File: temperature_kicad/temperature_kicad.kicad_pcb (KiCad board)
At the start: 2 copper layers, 35.6 x 30.5 mm, 13 parts, among them U1 nRF24L01, U2 DS18B20, U3 LD2980, U4 ATTINY13A-PU

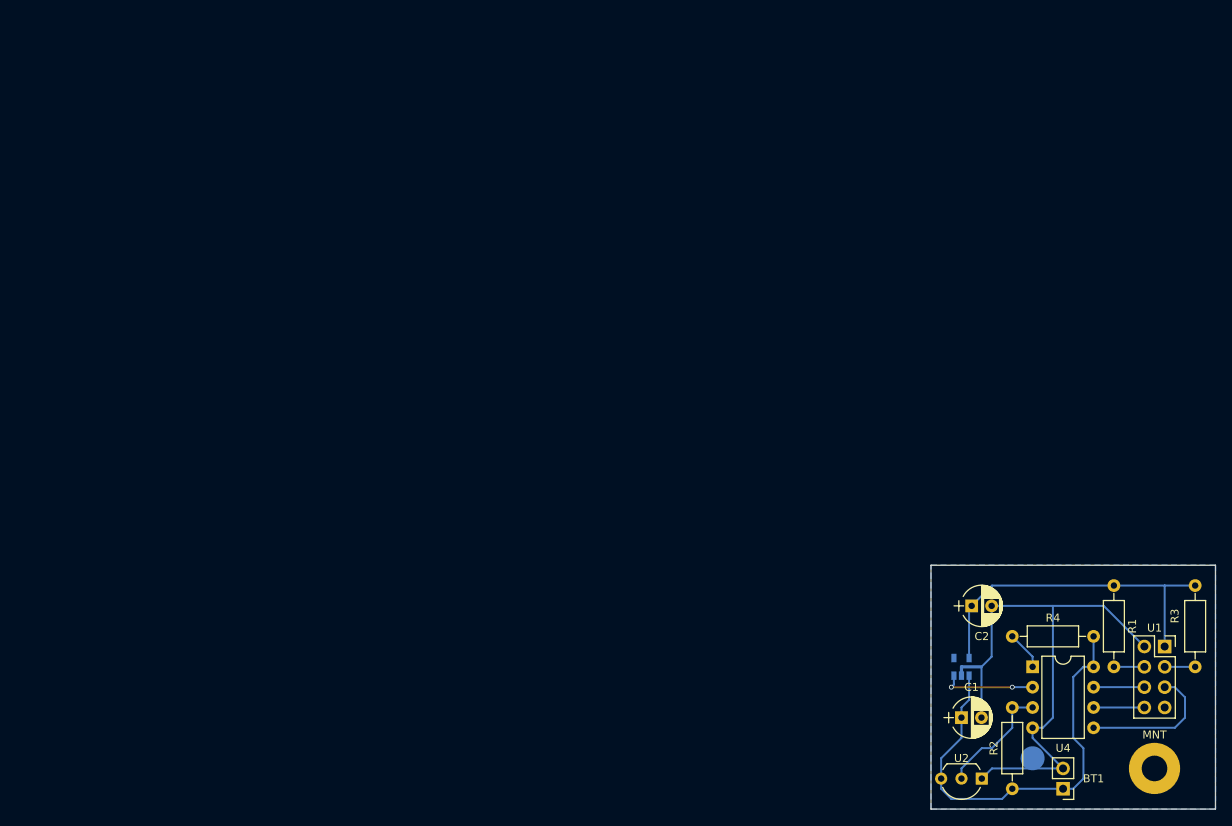
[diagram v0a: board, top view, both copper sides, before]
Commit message: Redone routing
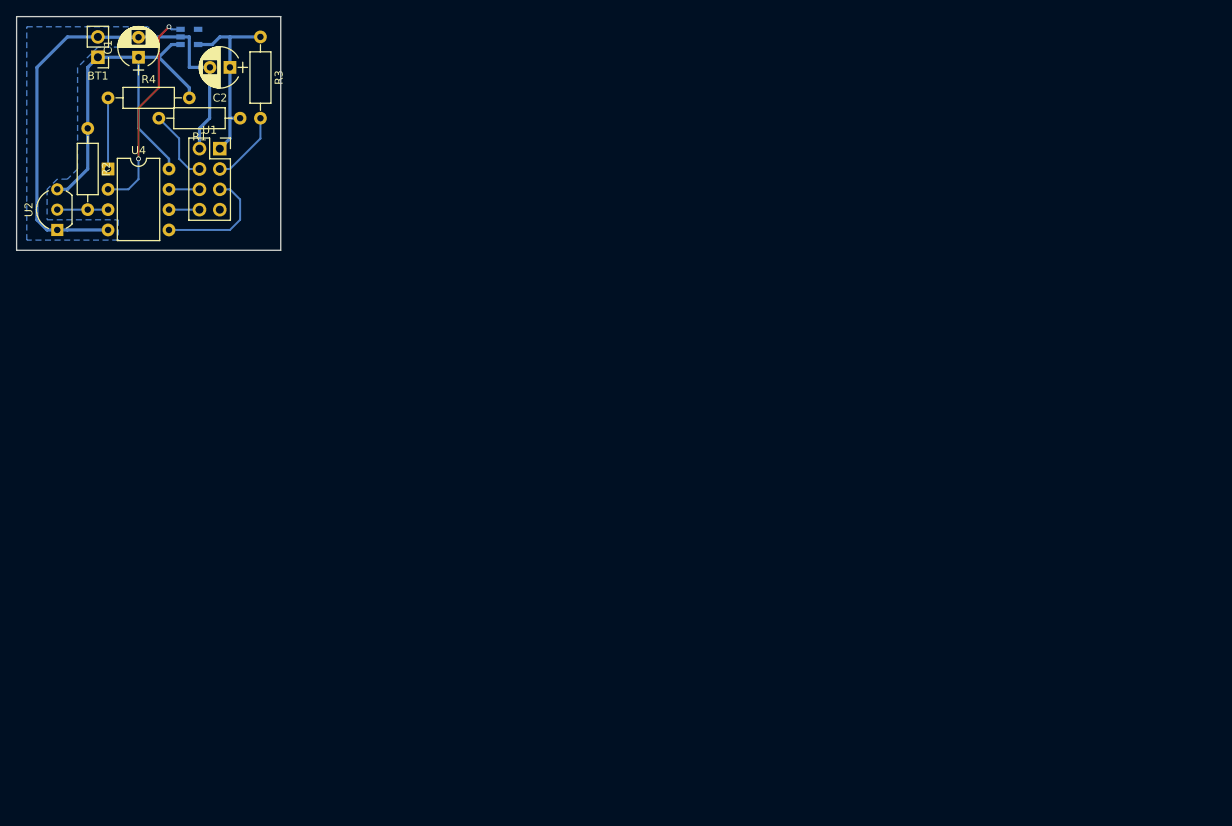
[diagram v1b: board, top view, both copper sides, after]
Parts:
- removed MNT: MountingHole_3.2mm_M3_Pad, Mounting_Holes:MountingHole_3.2mm_M3_Pad
- removed THERM: Measurement_Point_Round-SMD-Pad_Big, Measurement_Points:Measurement_Point_Round-SMD-Pad_Big
- moved BT1 151.4 mm to (20.3, 15.2)
- moved R2 142.0 mm to (19.1, 24.1), turned to 270 degrees
- moved R3 135.5 mm to (40.6, 12.7)
- moved U2 134.4 mm to (15.2, 36.8), turned to 90 degrees
- moved U1 133.5 mm to (35.6, 26.7)
- moved C1 131.9 mm to (25.4, 15.2), turned to 90 degrees
- moved R4 131.6 mm to (21.6, 20.3)
- moved U4 131.3 mm to (21.6, 29.2)
- moved U3 124.6 mm to (31.8, 12.7), turned to 0 degrees
- moved R1 123.9 mm to (38.1, 22.9), turned to 180 degrees
- moved C2 114.6 mm to (36.8, 16.5), turned to 180 degrees
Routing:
- net VDD: track 43.3 -> 23.9 mm
- net TR_EN: track 11.7 -> 26.5 mm
- net Net-(R2-Pad2): track 14.8 -> 6.35 mm
- net GND: track 73.7 -> 66.4 mm
- net Net-(R1-Pad2): track 3.81 -> 9.20 mm
- net Net-(R3-Pad2): track 3.81 -> 9.20 mm
- net Net-(R4-Pad1): track 4.86 -> 8.89 mm
- net Net-(U1-Pad5): track 17.6 -> 15.0 mm
- net Net-(U1-Pad8): track 6.35 -> 3.81 mm
- net Net-(U1-Pad6): track 6.35 -> 3.81 mm
- net VCC: track 55.0 -> 52.6 mm
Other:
- board size 35.6 x 30.5 mm -> 33 x 29.2 mm
- net class Ground removed
- net class Power added: clearance 0.2, trace_width 0.4, via_dia 0.6, via_drill 0.4
